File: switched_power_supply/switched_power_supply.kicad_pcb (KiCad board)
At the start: 2 copper layers, 80 x 80 mm, 35 parts, among them IC1 VIPER53ESPTR-E, T1 Transformador_1x2, U2 TL431, U3 PC817 Opto

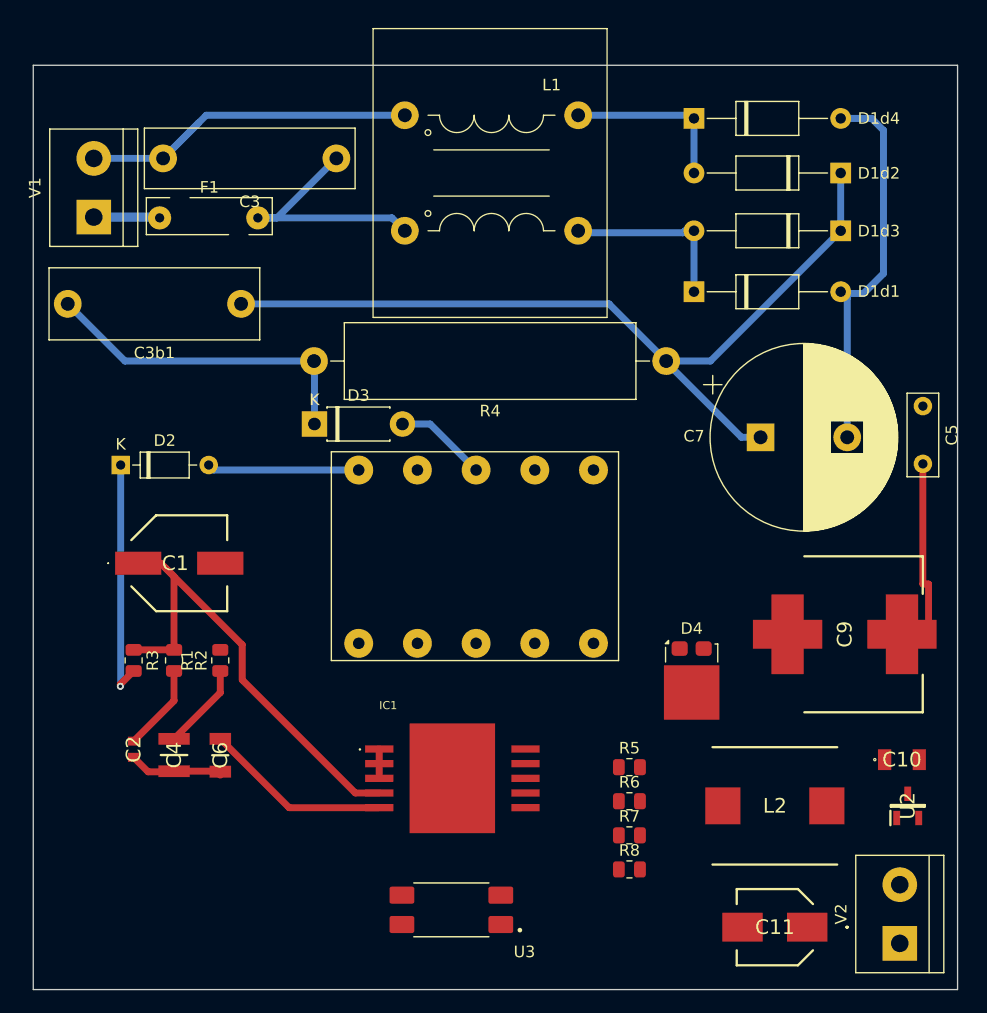
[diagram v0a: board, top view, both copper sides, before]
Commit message: pcb atualizado
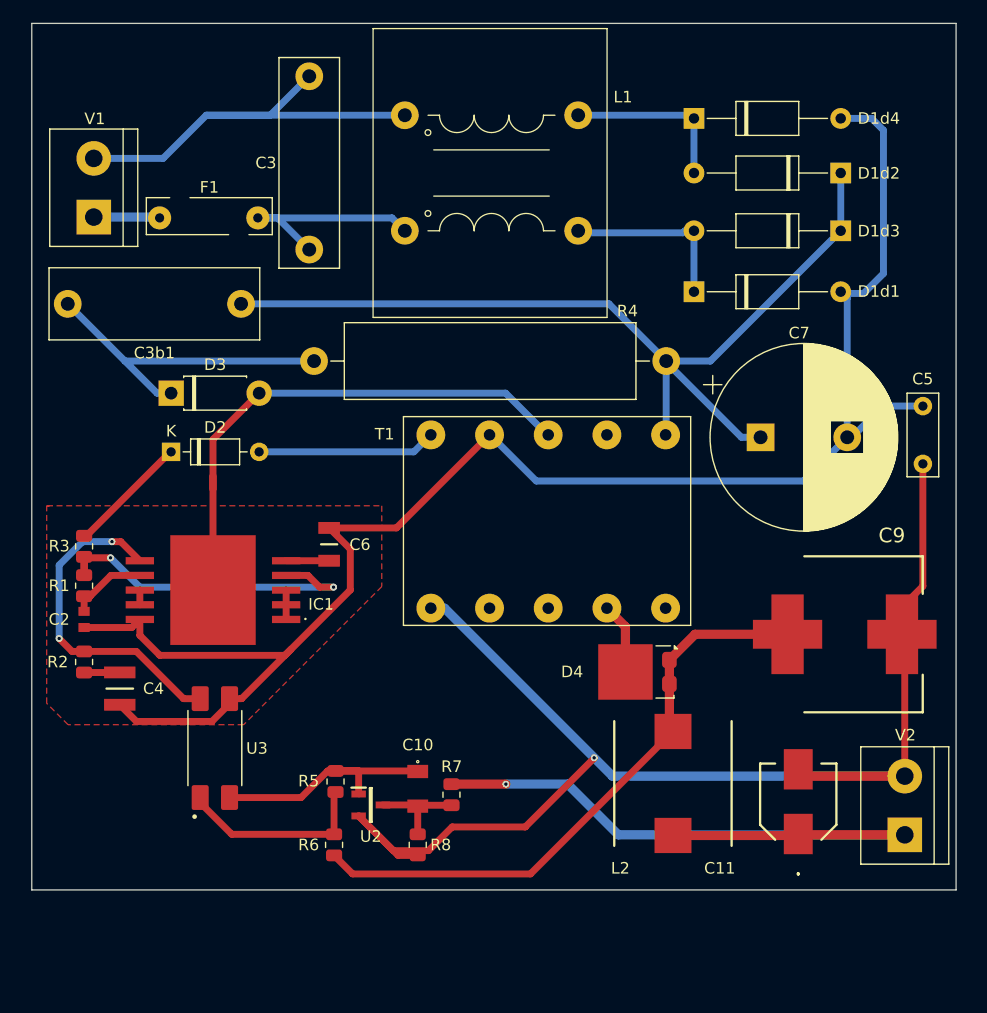
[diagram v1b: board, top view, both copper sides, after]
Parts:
- removed C1: Capacitor_Eletrolitico, pci:EEHZT1E331UP
- moved U2 46.5 mm to (136.0, 116.9), turned to 0 degrees
- moved C10 42.0 mm to (140.1, 115.5), turned to -90 degrees
- moved IC1 26.4 mm to (122.4, 98.3), turned to 180 degrees
- moved R6 25.8 mm to (132.8, 120.4), turned to 90 degrees
- moved R5 25.5 mm to (133.0, 114.9), turned to 90 degrees
- moved U3 24.8 mm to (122.5, 112.0), turned to 90 degrees
- moved C6 20.5 mm to (132.4, 94.4), turned to 90 degrees
- moved R8 18.4 mm to (140.1, 120.4), turned to -90 degrees
- moved R7 15.8 mm to (143.0, 116.0), turned to -90 degrees
- moved D3 12.7 mm to (118.7, 81.3)
- moved C2 12.0 mm to (111.2, 100.9)
- moved R2 11.8 mm to (111.2, 104.5)
- moved C11 11.1 mm to (173.0, 116.6), turned to 90 degrees
- moved R3 10.8 mm to (111.2, 94.5), turned to 90 degrees
- moved R1 10.1 mm to (111.2, 97.9)
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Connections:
- D4 pad 3: (no net) -> Net-(D4-A)
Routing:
- net GND: track 42.0 -> 145.1 mm
- net Terra: track 18.0 -> 113.0 mm, vias 0 -> 1
- net /Vout: track 0.00 -> 61.2 mm, vias 0 -> 1
- net Net-(D4-K): track 0.00 -> 52.6 mm
- net /Drain: track 8.02 -> 46.4 mm
- net /Cmp: track 0.00 -> 29.2 mm, vias 0 -> 2
- net Net-(U3-Cath): track 0.00 -> 21.3 mm
- net Net-(U3-Anode): track 0.00 -> 17.4 mm
- net /TOVL: track 16.2 -> 3.85 mm
- net /Vdd: track 41.8 -> 30.2 mm, vias 0 -> 2
- net Net-(D2-K): track 21.0 -> 10.5 mm, vias 1 -> 0
- net Net-(C10-Pad2): track 0.00 -> 8.45 mm
- net Net-(D4-A): track 0.00 -> 6.19 mm
- net Net-(C3-Pad2): track 32.9 -> 38.9 mm
- net /BarP: track 75.8 -> 81.3 mm
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- added copper zone on F.Cu, net GND
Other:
- board size 80 x 80 mm -> 80 x 75 mm
